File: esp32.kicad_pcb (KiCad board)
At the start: 2 copper layers, 25.4 x 41.4 mm, 23 parts, among them IC1 ESP32-WROVER-E_M213EH6464PH3Q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, J1 Micro_SD_Card_Det, J2 Conn_01x10_Male, J3 Conn_01x10_Male, Q1 UMH3N, U1 MCP2518FDT-H_SL, U2 SN65HVD231, Y1 XRCGB40M000F4M02R0

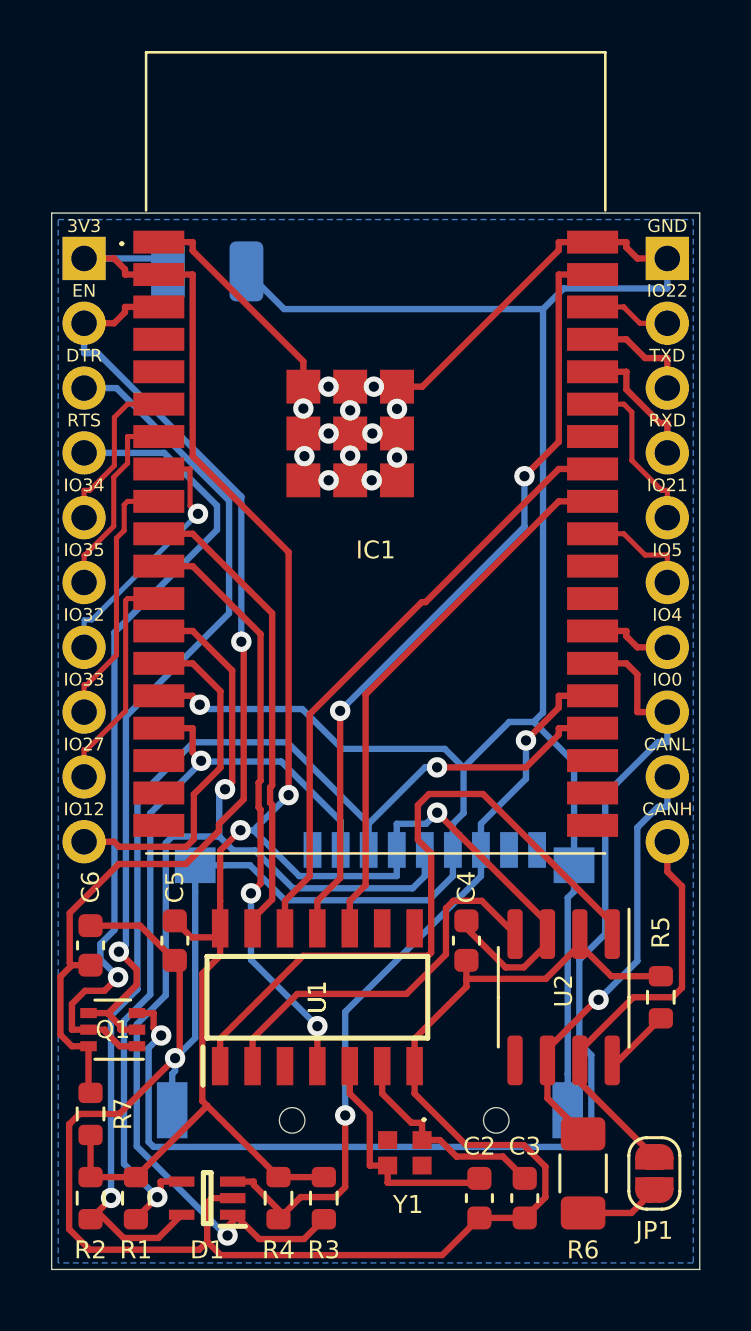
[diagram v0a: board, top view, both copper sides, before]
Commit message: Alle ESP Pins
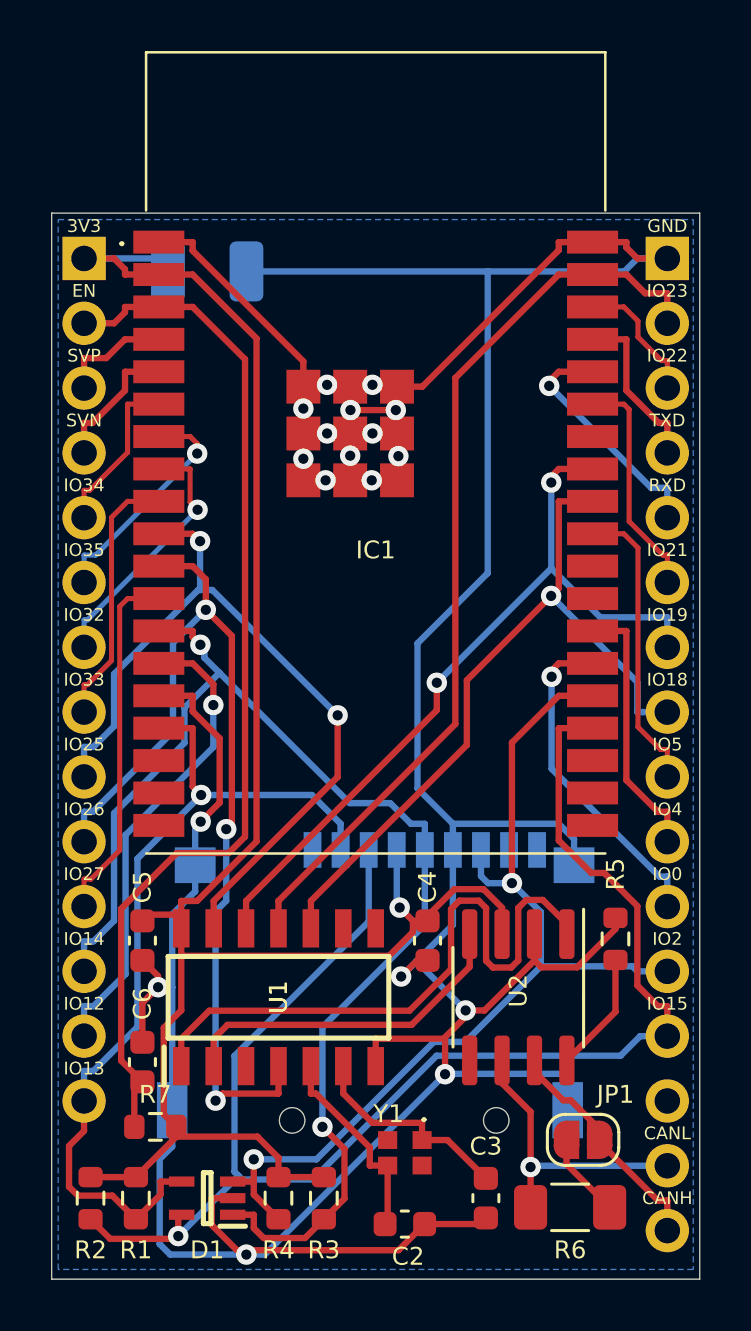
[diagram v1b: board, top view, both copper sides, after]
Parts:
- removed Q1: UMH3N, Package_TO_SOT_SMD:SOT-363_SC-70-6
- J2: value Conn_01x10_Male -> Conn_01x14_Male; footprint Connector_PinHeader_2.54mm:PinHeader_1x10_P2.54mm_Vertical -> Connector_PinHeader_2.54mm:PinHeader_1x14_P2.54mm_Vertical
- J3: value Conn_01x10_Male -> Conn_01x16_Male; footprint Connector_PinHeader_2.54mm:PinHeader_1x10_P2.54mm_Vertical -> Connector_PinHeader_2.54mm:PinHeader_1x16_P2.54mm_Vertical
- moved C6 5.00 mm to (88.6, 97.5)
- moved C2 3.09 mm to (98.9, 103.9), turned to 180 degrees
- moved JP1 3.09 mm to (105.9, 100.6), turned to 180 degrees
- moved R5 2.90 mm to (107.2, 92.7)
- moved R7 2.59 mm to (89.2, 100.1), turned to 180 degrees
- moved U2 1.78 mm to (103.4, 95.0)
- moved C3 1.52 mm to (102.1, 102.9)
- moved C4 1.52 mm to (99.8, 92.8)
- moved U1 1.52 mm to (94.0, 95.0)
- moved R6 1.42 mm to (105.4, 103.2), turned to 180 degrees
- moved C5 1.27 mm to (88.6, 92.8)
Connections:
- J2 pad 10: Net-(IC1-Pad14) -> MCP_INT
- J2 pad 3: DTR -> Net-(IC1-Pad4)
- J2 pad 4: RTS -> Net-(IC1-Pad5)
- J2 pad 9: Net-(IC1-Pad12) -> MCP_CS
- J3 pad 10: CANH -> Net-(IC1-Pad26)
- J3 pad 2: Net-(IC1-Pad36) -> MCP_MOSI
- J3 pad 3: TXD -> Net-(IC1-Pad36)
- J3 pad 4: RXD -> TXD
- J3 pad 5: Net-(IC1-Pad33) -> RXD
- J3 pad 6: Net-(IC1-Pad29) -> Net-(IC1-Pad33)
- J3 pad 7: Net-(IC1-Pad26) -> MCP_MISO
- J3 pad 8: IO0 -> MCP_CLK
- J3 pad 9: CANL -> Net-(IC1-Pad29)
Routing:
- net IO0: track 46.8 -> 13.0 mm
- net RTS: track 32.8 -> 0.00 mm, vias 1 -> 0
- net DTR: track 32.4 -> 0.00 mm, vias 1 -> 0
- net GND: track 198.3 -> 172.2 mm, vias 14 -> 18
- net MCP_INT: track 23.3 -> 38.1 mm, vias 2 -> 3
- net SD_CMD: track 44.1 -> 58.2 mm, vias 2 -> 1
- net MCP_CS: track 18.5 -> 30.9 mm, vias 0 -> 2
- net SD_DAT0: track 29.8 -> 38.5 mm
- net MCP_CLK: track 21.5 -> 29.2 mm, vias 0 -> 1
- net Net-(IC1-Pad29): track 4.35 -> 11.6 mm
- net Net-(IC1-Pad26): track 3.32 -> 10.5 mm
- net CANH: track 16.4 -> 9.21 mm
- net MCP_MISO: track 23.9 -> 30.9 mm, vias 0 -> 2
- net SD_CLK: track 45.0 -> 50.4 mm
- net Net-(IC1-Pad5): track 0.00 -> 5.37 mm
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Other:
- board size 25.4 x 41.4 mm -> 25.4 x 41.8 mm
- board text added: "IO13"
- board text added: "IO14"
- board text added: "IO15"
- board text added: "IO18"
- board text added: "IO19"
- board text added: "IO2"
- board text added: "IO23"
- board text added: "IO25"
- board text added: "IO26"
- board text added: "SVN"
- board text added: "SVP"
- board text removed: "DTR"
- board text removed: "RTS"
